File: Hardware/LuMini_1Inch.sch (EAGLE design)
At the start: 35 parts, among them J1 DOUBLE_LED_PAD, J2 DOUBLE_LED_PAD, J4 DOUBLE_LED_PAD

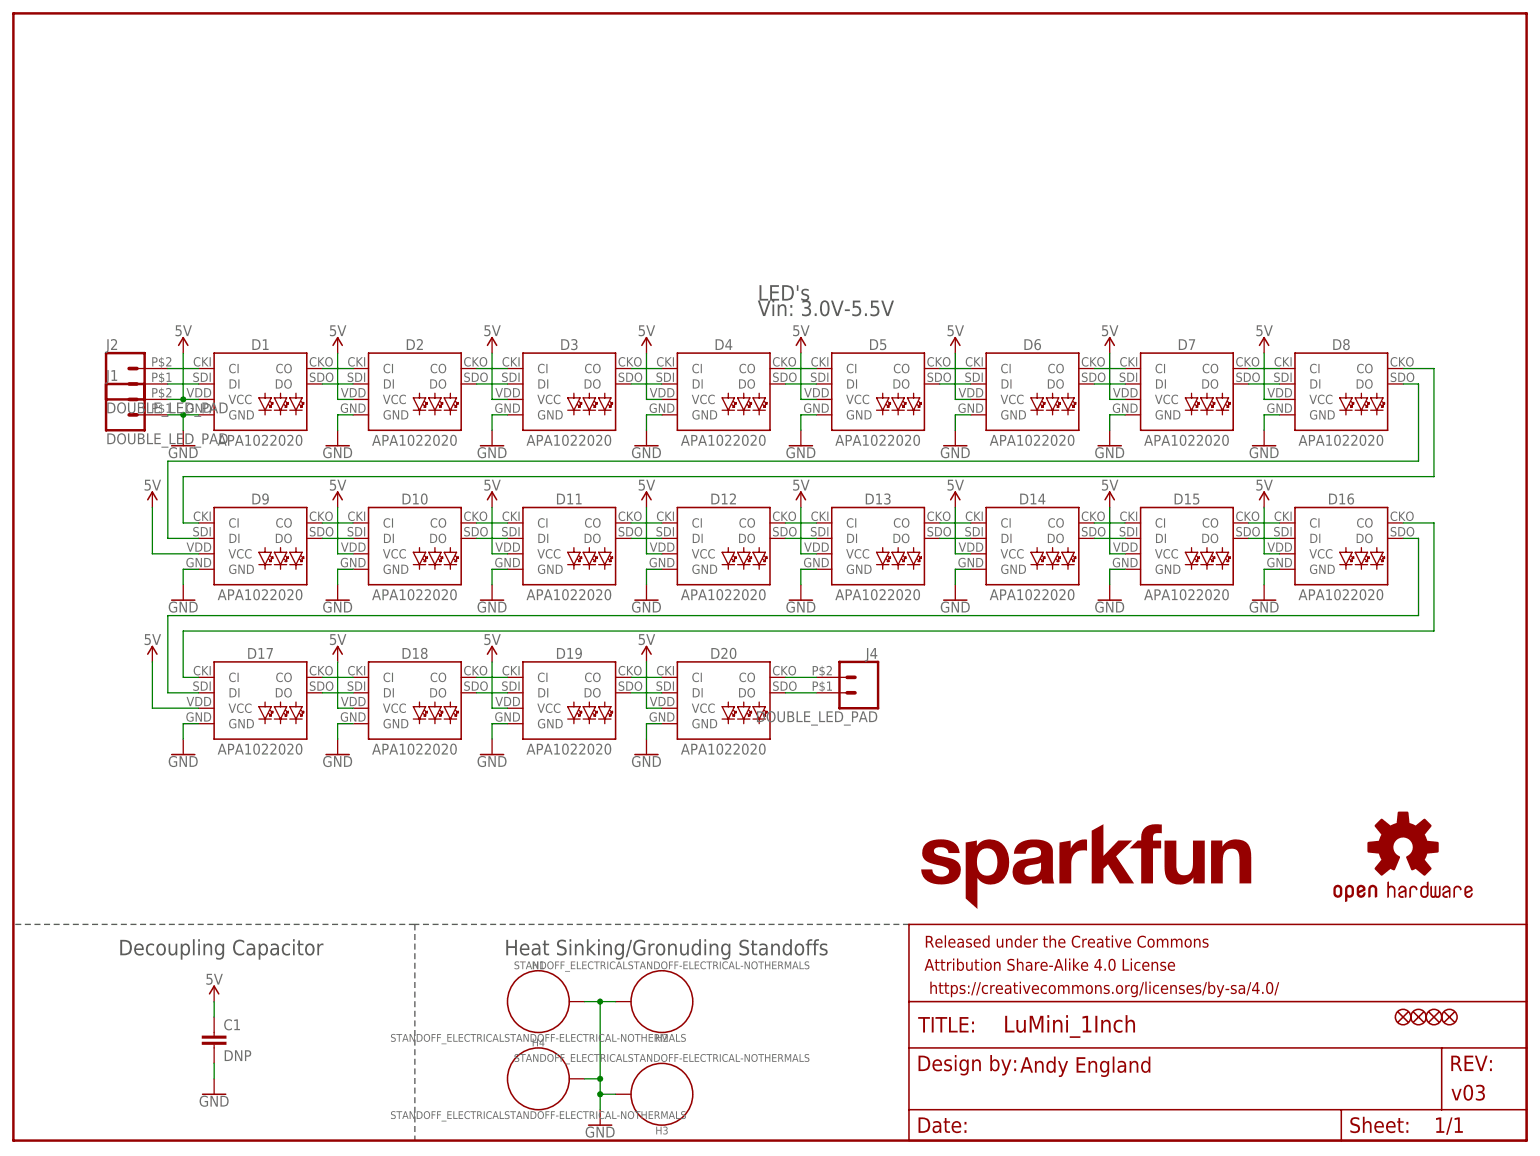
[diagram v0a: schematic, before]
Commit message: qc checklist changes
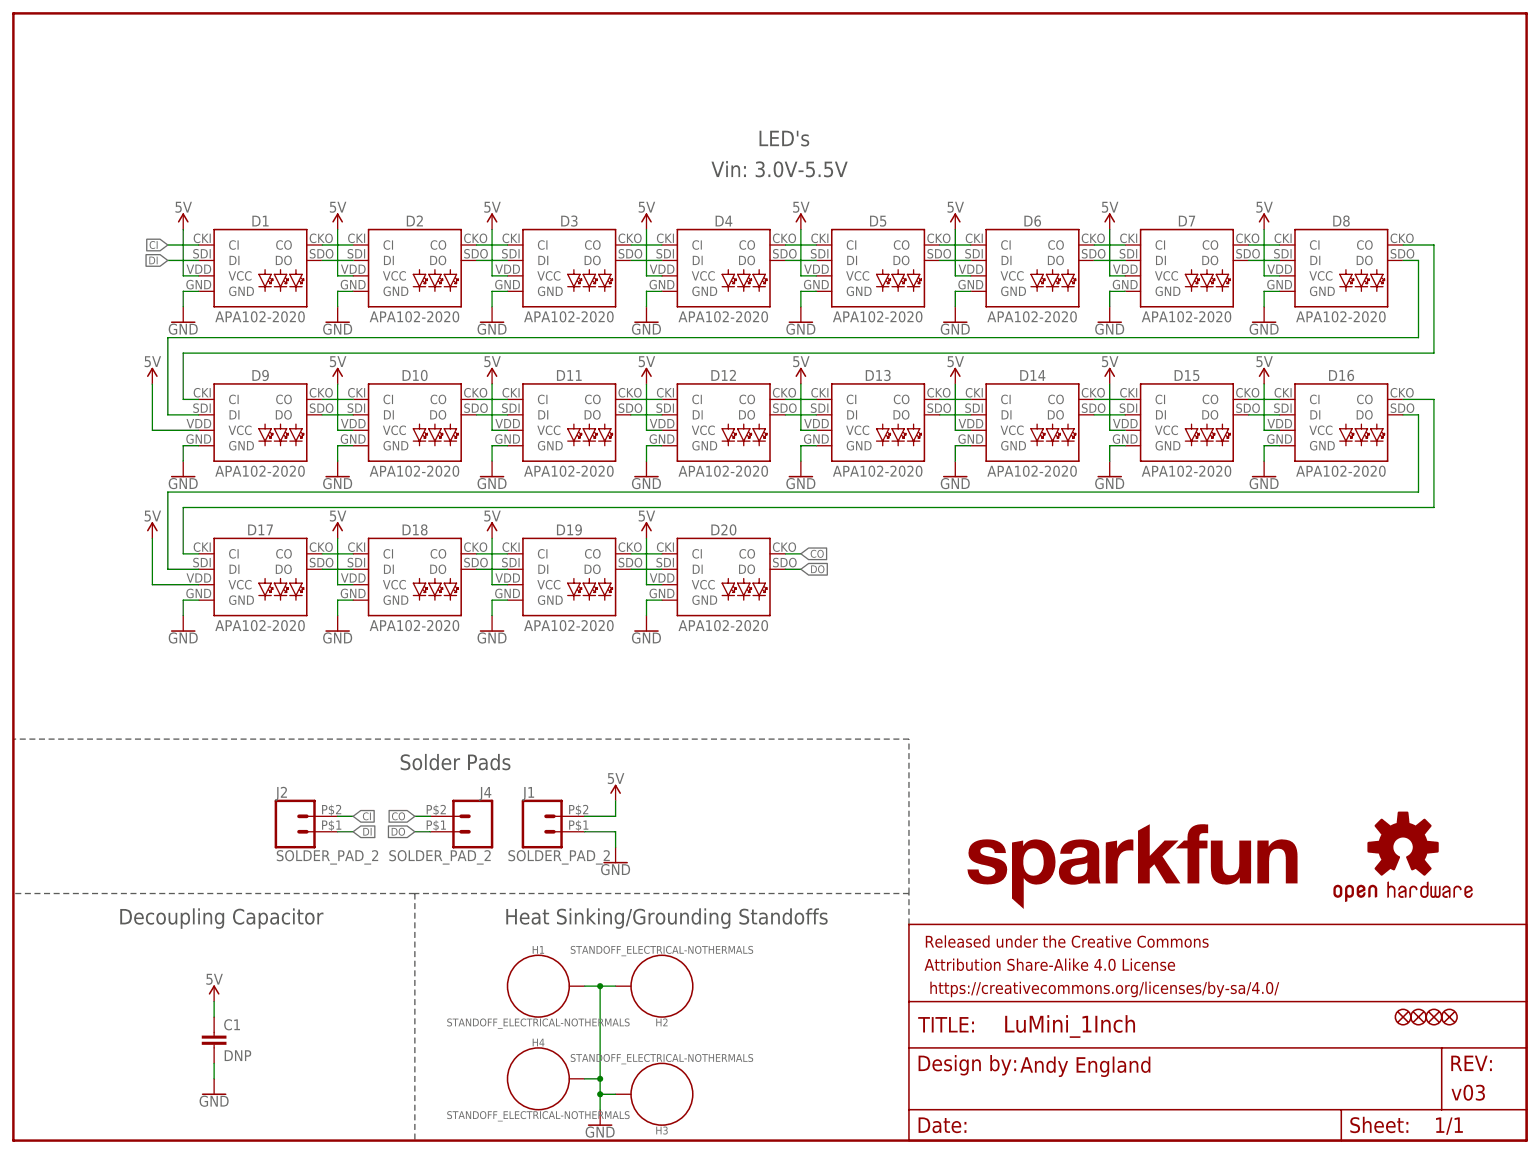
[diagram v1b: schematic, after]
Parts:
- D1, D10, D11, D12, D13, D14, D15, D16, D17, D18, D19, D2, D20, D3, D4, D5, D6, D7, D8, D9: value APA1022020 -> APA102-2020; device SparkFun-LED:APA1022020 -> SparkFun-LED:APA102-2020
- H1, H2, H3, H4: value STANDOFF_ELECTRICALSTANDOFF-ELECTRICAL-NOTHERMALS -> STANDOFF_ELECTRICAL-NOTHERMALS; device SparkFun-Hardware:STANDOFF_ELECTRICALSTANDOFF-ELECTRICAL-NOTHERMALS -> SparkFun-Hardware:STANDOFF_ELECTRICAL-NOTHERMALS
- J1, J2, J4: value DOUBLE_LED_PAD -> SOLDER_PAD_2; device Andy:DOUBLE_LED_PAD -> SparkFun-Connectors:SOLDER_PAD_2
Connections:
- net N$2 renamed CI
- net N$3 renamed DI
- net N$41 renamed CO
- net N$42 renamed DO
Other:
- note added: "Heat Sinking/Grounding Standoffs"
- note added: "Solder Pads"
- note removed: "Heat Sinking/Gronuding Standoffs"
- moved on the sheet: D1, D10, D11, D12, D13, D14, D15, D16, D17, D18, D19, D2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
